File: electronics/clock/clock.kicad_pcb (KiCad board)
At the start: 2 copper layers, 109.2 x 61 mm, 51 parts, among them J1 Conn_02x03_Counter_Clockwise, J2 Conn_01x02_Male, Q1 2SC1815, Q2 2SC1815, Q3 2SC1815, Q4 2SC1815, Q5 2SC1815, SW2 SW_Push, SW3 SW_Push, SW4 SW_Push, SW5 SW_Push, SW6 SW_Push, SW7 SW_Push, SW8 SW_Push, SW9 SW_Push, U1 ATtiny2313-20P, U2 74HC595, U3 74HC165, Y1 Crystal

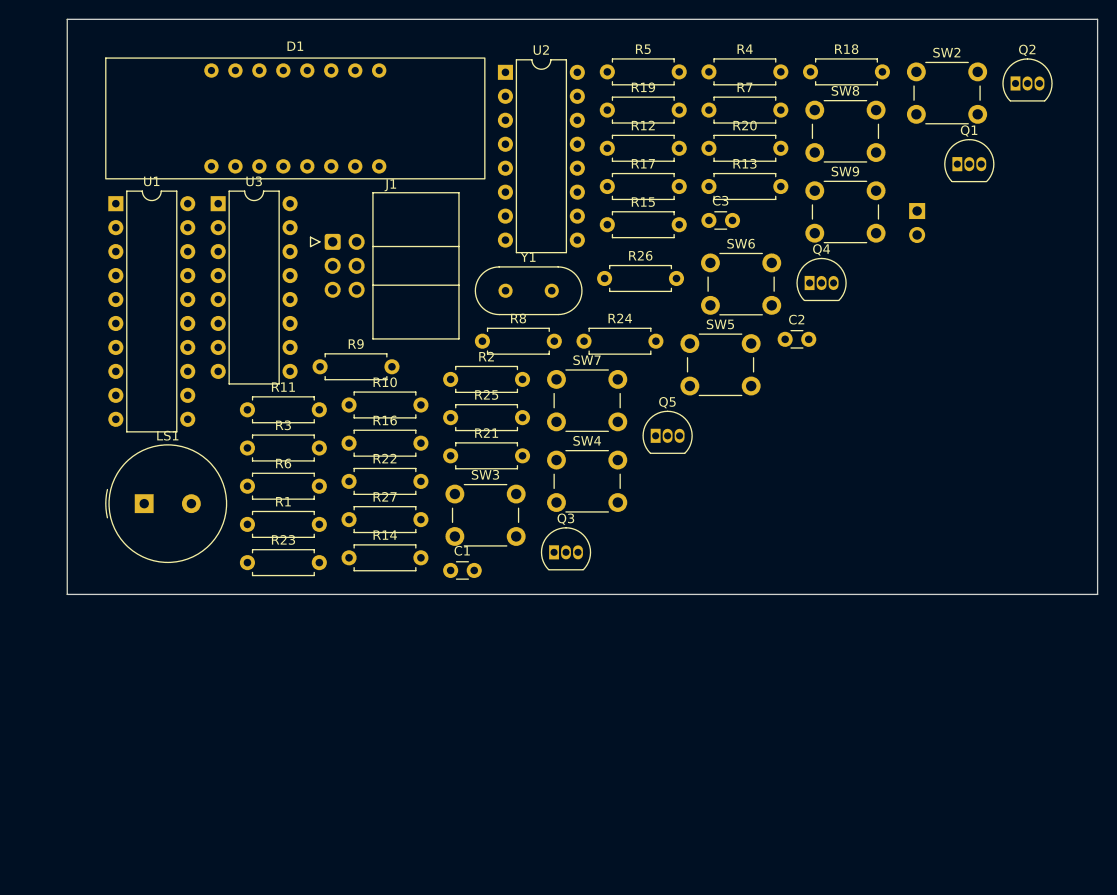
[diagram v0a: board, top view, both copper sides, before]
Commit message: [update] v0.0.1を作成
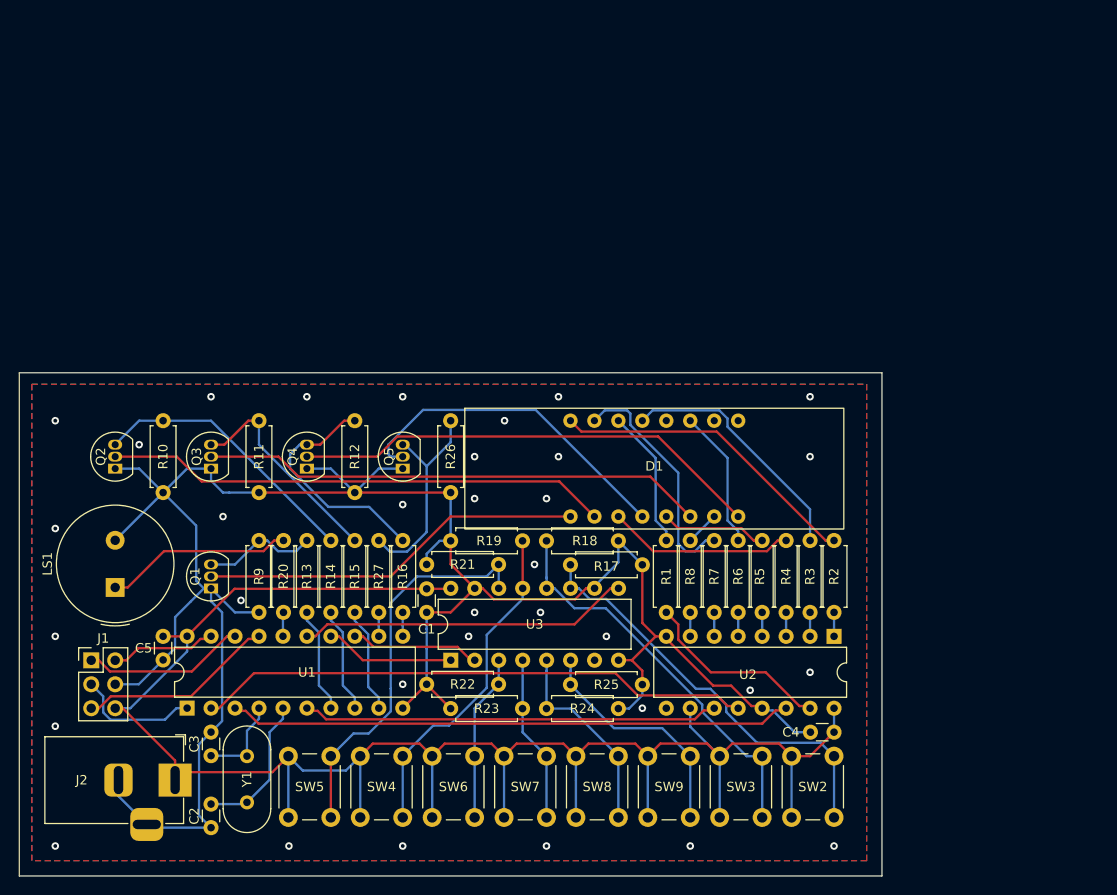
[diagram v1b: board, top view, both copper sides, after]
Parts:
- added C4: 0.1u, Capacitor_THT:C_Disc_D3.0mm_W1.6mm_P2.50mm, F.Cu at (180.3, 118.7)
- added C5: 0.1u, Capacitor_THT:C_Disc_D3.0mm_W1.6mm_P2.50mm, F.Cu at (109.2, 108.6)
- J1: footprint Connector_IDC:IDC-Header_2x03_P2.54mm_Horizontal -> Connector_PinHeader_2.54mm:PinHeader_2x03_P2.54mm_Vertical
- J2: value Conn_01x02_Male -> Barrel_Jack_Switch; footprint Connector_PinSocket_2.54mm:PinSocket_1x02_P2.54mm_Vertical -> Connector_BarrelJack:BarrelJack_Horizontal; moved to F.Cu
- R1, R2, R3, R4, R5, R6, R7, R8: value 220 -> 330
- R10, R11, R12, R26, R9: value 47k -> 10k
- R13, R14, R15, R16, R27: value 2.2k -> 3.9k
- R17, R18, R19, R20, R21, R22, R23, R24, R25: value R -> 1k
- Y1: value Crystal -> 16 MHz
- moved Q2 103.8 mm to (104.1, 90.8), turned to 90 degrees
- moved J2 99.1 mm to (110.5, 123.8), turned to 0 degrees
- moved Q1 91.0 mm to (114.3, 103.5), turned to 90 degrees
- moved SW2 80.1 mm to (175.8, 127.8), turned to 90 degrees
- moved C2 79.9 mm to (114.3, 128.9), turned to 90 degrees
- moved SW8 79.1 mm to (153.0, 127.8), turned to 90 degrees
- moved C3 75.7 mm to (114.3, 118.7), turned to -90 degrees
- moved U2 69.2 mm to (180.3, 108.6), turned to -90 degrees
- moved SW9 68.8 mm to (160.6, 127.8), turned to 90 degrees
- moved R20 66.7 mm to (122.0, 106.0), turned to 90 degrees
- moved SW5 65.8 mm to (122.5, 127.8), turned to 90 degrees
- moved SW6 65.8 mm to (137.7, 127.8), turned to 90 degrees
- moved R3 62.1 mm to (177.8, 106.0), turned to 90 degrees
- moved Y1 60.8 mm to (118.1, 126.2), turned to 90 degrees
- moved R5 59.6 mm to (172.7, 106.0), turned to 90 degrees
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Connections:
- net +3V0 renamed +5V
- net 7seg-rclk renamed 7SEG_RCLK
- net 7seg-ser renamed 7SEG_SER
- net 7seg-srclk renamed 7SEG_SRCLK
- net dig-1 renamed DIG_1
- net dig-2 renamed DIG_2
- net dig-3 renamed DIG_3
- net dig-4 renamed DIG_4
- net dig-dot renamed DIG_DOT
- net isp-clk renamed ISP_CLK
- net isp-miso renamed ISP_MISO
- net isp-mosi renamed ISP_MOSI
- net isp-reset renamed ISP_RESET
- net sw-clk renamed SW_CLK
- net sw-out renamed SW_OUT
- net sw-s/l renamed SW_S/L
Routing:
- net GND: track 0.00 -> 234.6 mm, vias 0 -> 34
- net +5V: track 0.00 -> 195.4 mm
- net 7SEG_SER: track 0.00 -> 59.8 mm
- net 7SEG_RCLK: track 0.00 -> 58.9 mm
- net Net-(D1-Pad2): track 0.00 -> 53.4 mm
- net Net-(D1-Pad6): track 0.00 -> 53.4 mm
- net Net-(D1-Pad8): track 0.00 -> 50.1 mm
- net Net-(R17-Pad1): track 0.00 -> 44.7 mm
- net 7SEG_SRCLK: track 0.00 -> 44.2 mm
- net Net-(R18-Pad1): track 0.00 -> 42.2 mm
- net Net-(R21-Pad1): track 0.00 -> 42.0 mm
- net Net-(D1-Pad1): track 0.00 -> 40.7 mm
- net Net-(D1-Pad4): track 0.00 -> 35.8 mm
- net Net-(R19-Pad1): track 0.00 -> 35.6 mm
- net SW_OUT: track 0.00 -> 35.1 mm
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- added copper zone on B.Cu, net GND
- added copper zone on F.Cu, net GND
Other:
- board size 109.2 x 61 mm -> 91.4 x 53.3 mm
- board text added: "github.com/shimo8810/diy-clock v0.0.1"
